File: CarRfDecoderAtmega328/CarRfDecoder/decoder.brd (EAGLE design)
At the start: 98.7 x 80 mm, 53 parts, among them T1 BC847, T2 BC847, T3 IRLML6402, U2 RFM69CW, U3 MCP73831, U4 ATMEGA328P, U6 MIC5219 3.3V, Y1 16MHZ

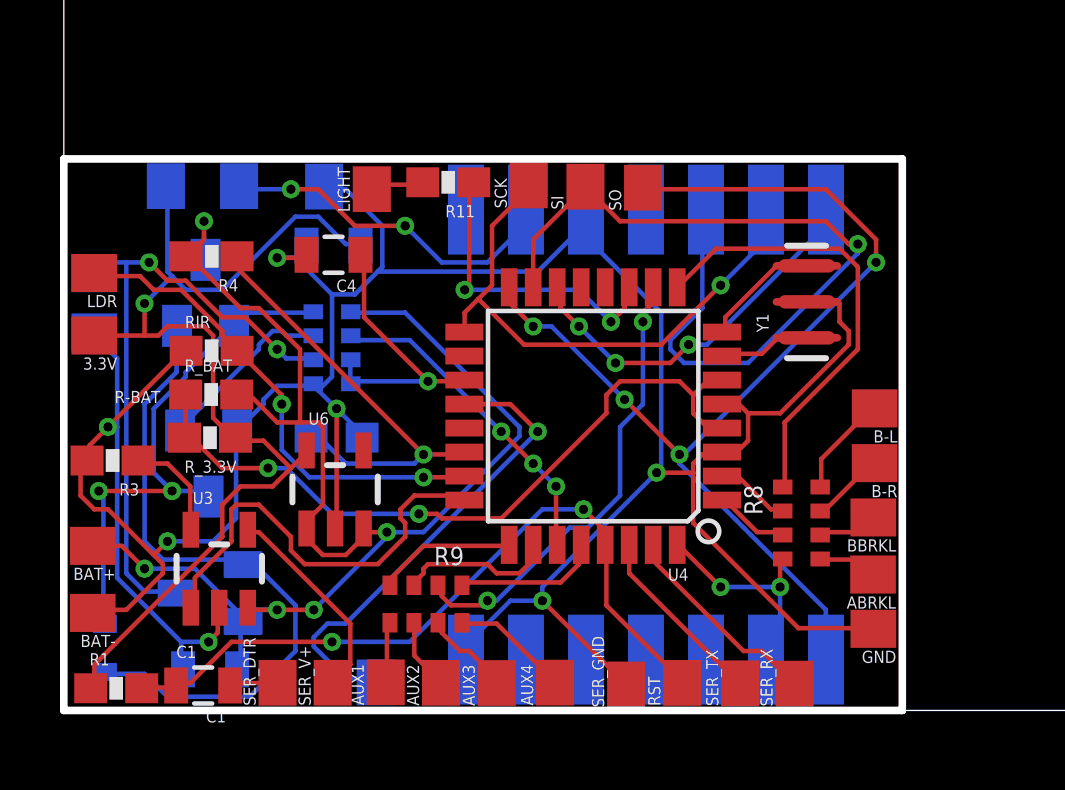
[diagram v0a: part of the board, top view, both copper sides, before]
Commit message: small fixes for vcc.
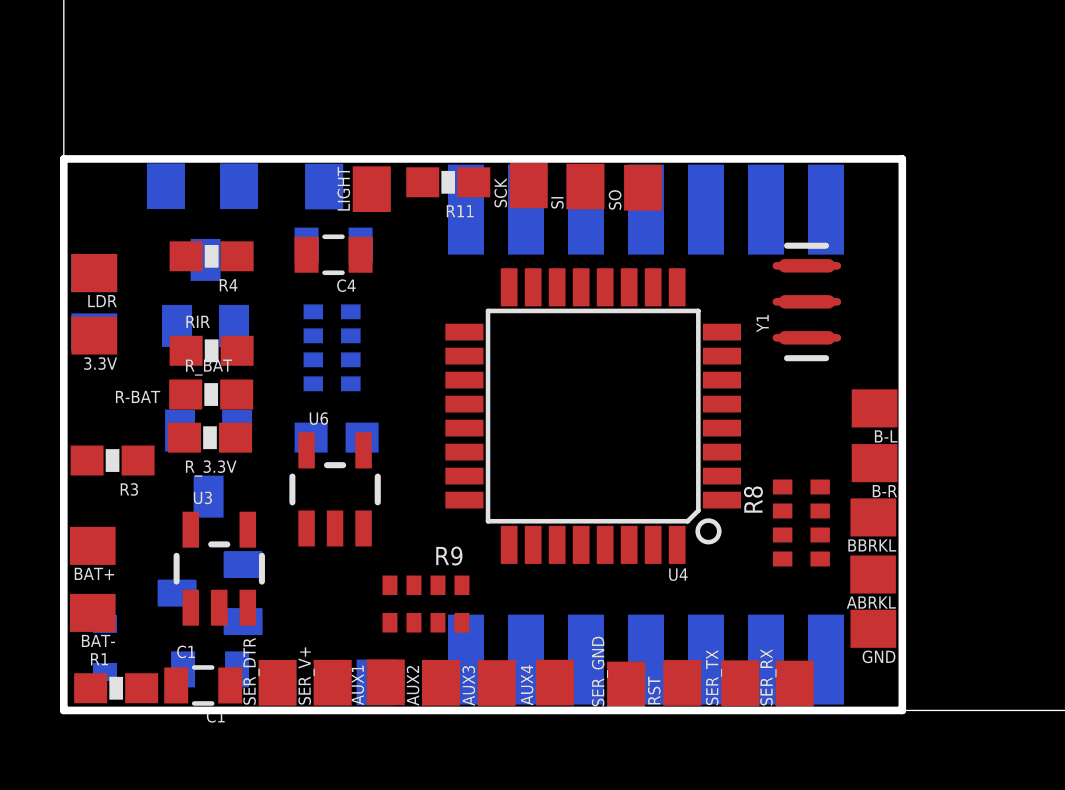
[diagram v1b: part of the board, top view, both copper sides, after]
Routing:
- net GND: track 111.4 -> 0.00 mm, vias 7 -> 0
- net BAT+: track 49.5 -> 0.00 mm, vias 5 -> 0
- net MISO: track 35.6 -> 0.00 mm, vias 4 -> 0
- net VCC: track 35.2 -> 0.00 mm, vias 1 -> 0
- net MOSI: track 27.4 -> 0.00 mm, vias 1 -> 0
- net N$6: track 24.9 -> 0.00 mm, vias 2 -> 0
- net N$5: track 24.4 -> 0.00 mm, vias 2 -> 0
- net N$14: track 22.4 -> 0.00 mm
- net N$15: track 21.2 -> 0.00 mm, vias 2 -> 0
- net SCK: track 18.5 -> 0.00 mm, vias 1 -> 0
- net N$19: track 18.0 -> 0.00 mm, vias 2 -> 0
- net A0: track 16.4 -> 0.00 mm, vias 2 -> 0
- net AREF: track 16.0 -> 0.00 mm, vias 1 -> 0
- net D6: track 15.4 -> 0.00 mm, vias 2 -> 0
- net BL: track 15.2 -> 0.00 mm
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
